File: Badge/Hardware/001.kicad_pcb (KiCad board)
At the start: 2 copper layers, 92.2 x 84.3 mm, 3 parts

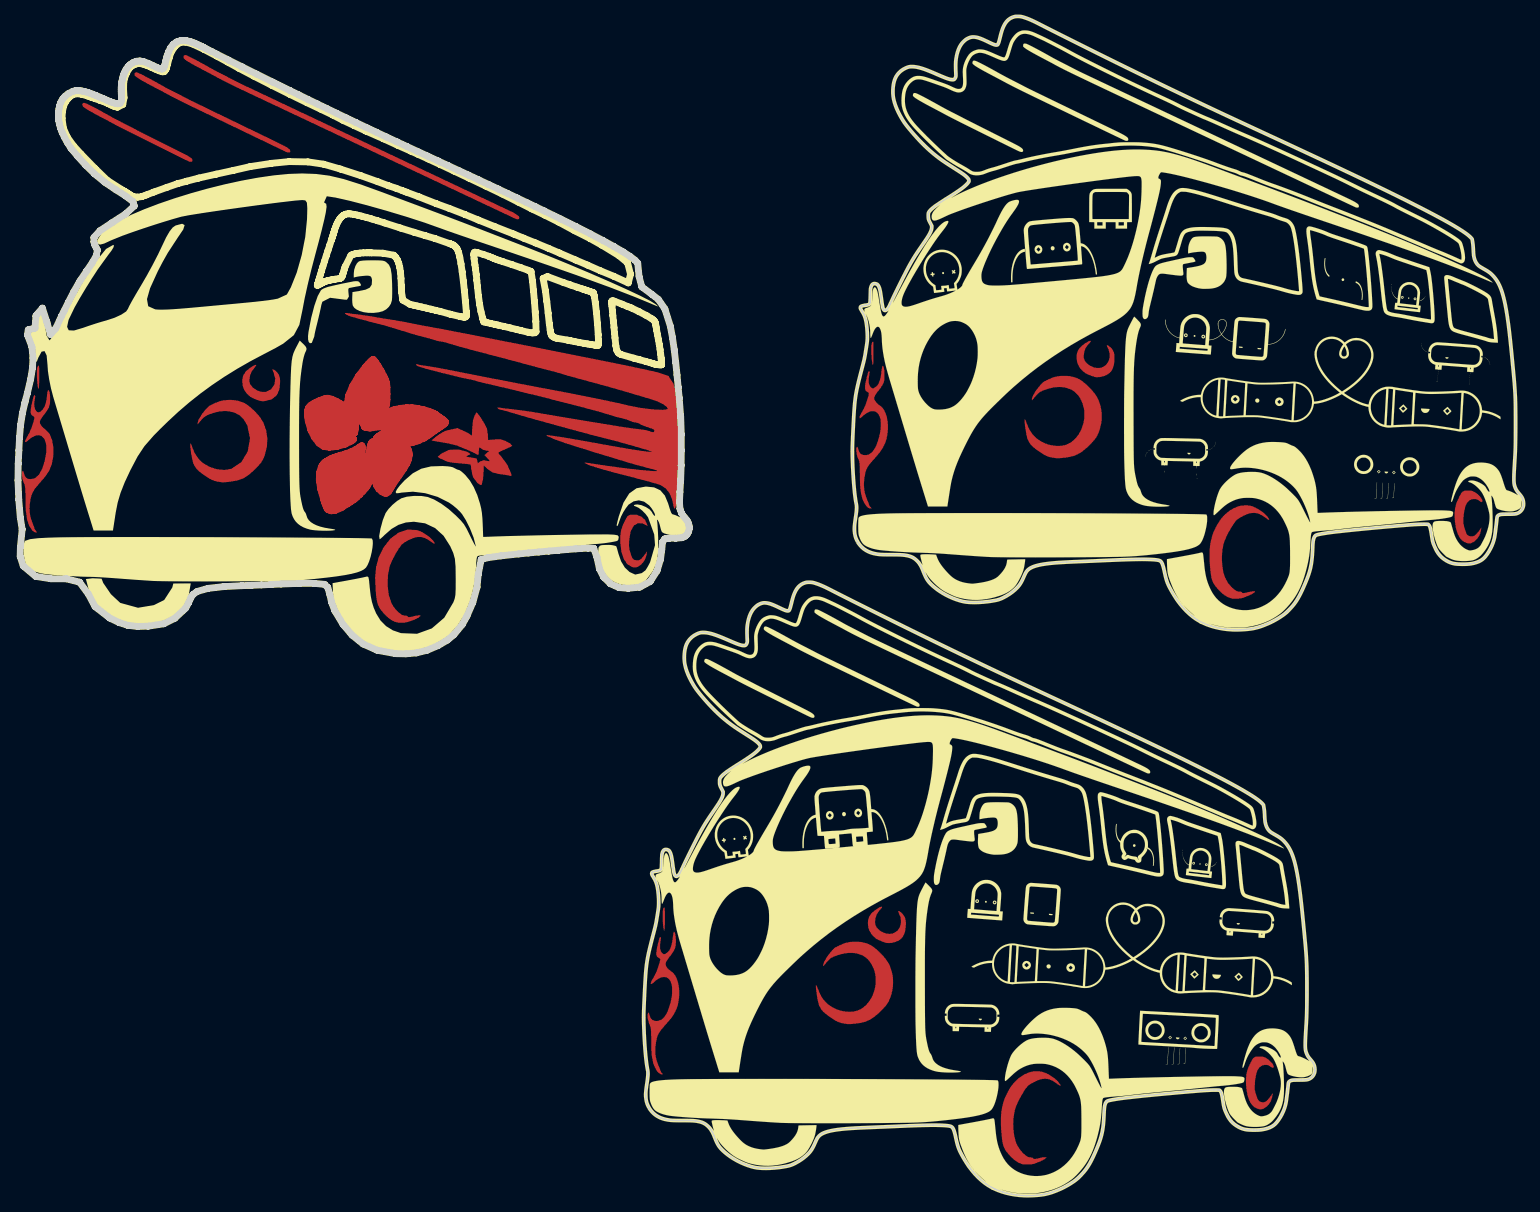
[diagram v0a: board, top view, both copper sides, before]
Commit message: Updates
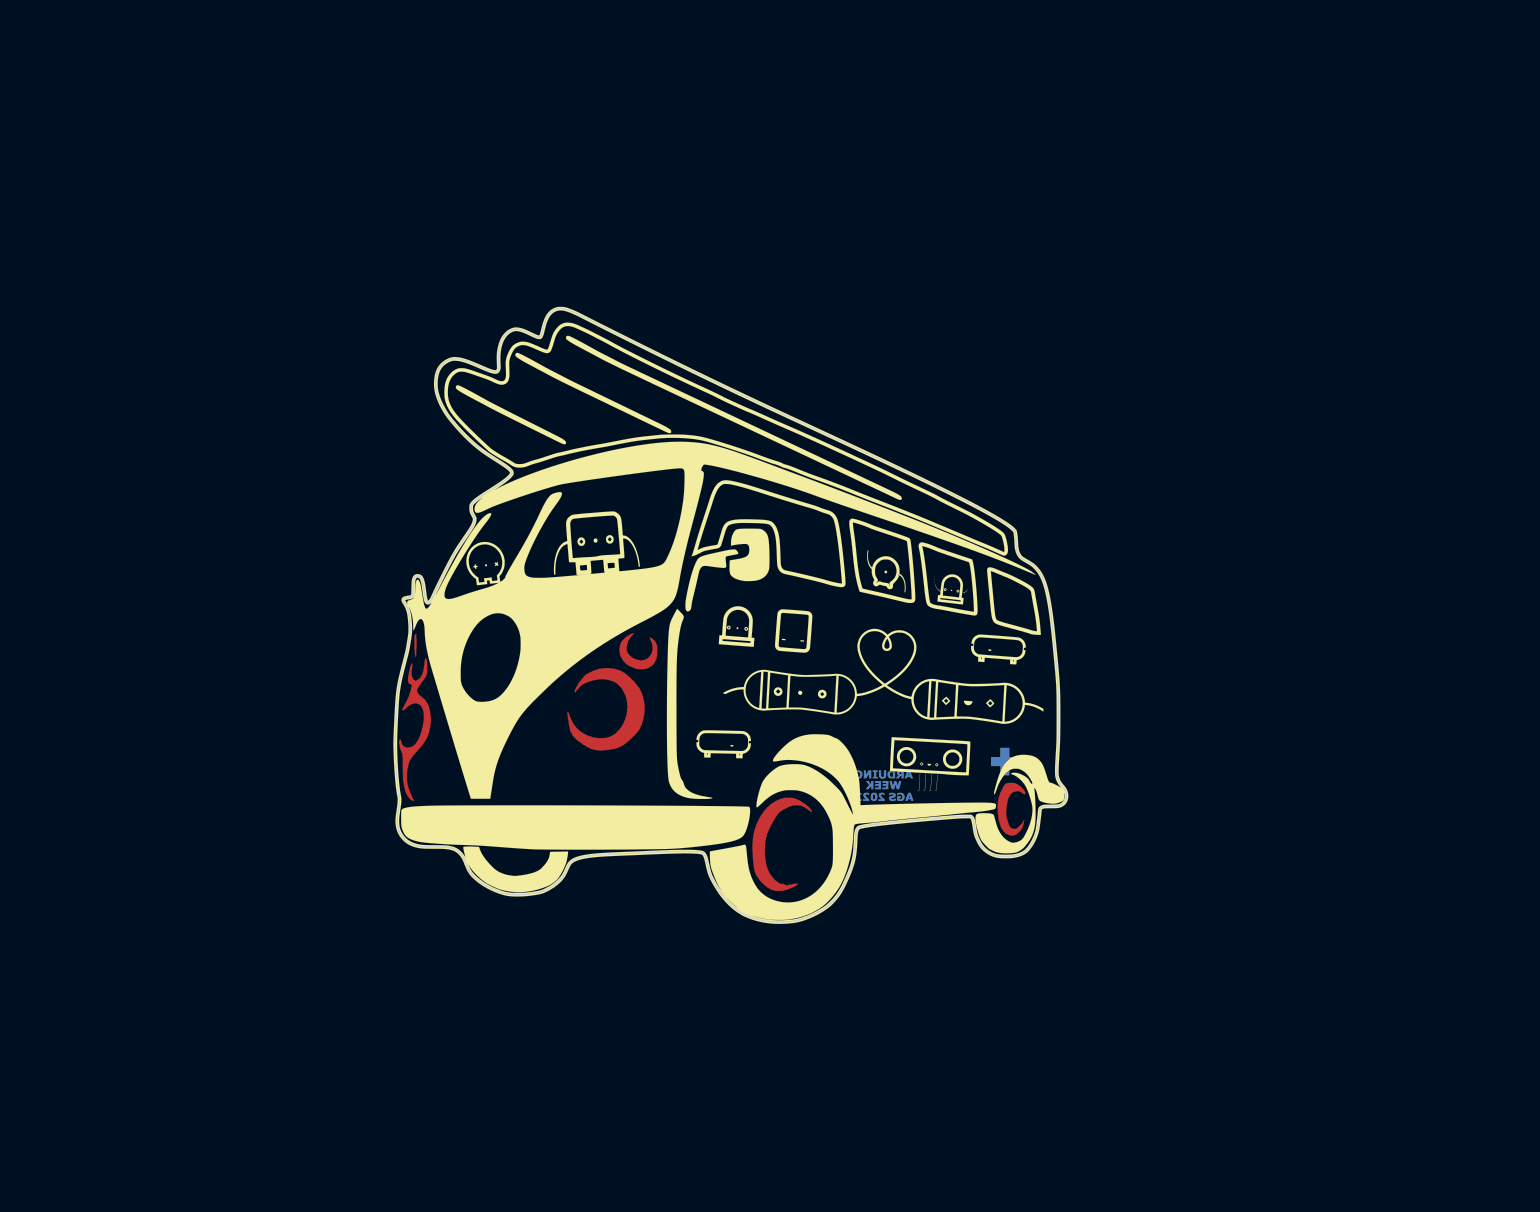
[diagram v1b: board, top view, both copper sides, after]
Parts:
- removed the Ref** at (203.7, 55.1)
- removed svg2mod: G***, combi:Combi.All.03
- added Ref**: Val**, combi:logo_AGS_2022, F.Cu at (172.7, 118.1)
- moved Ref** 50.7 mm to (141.0, 95.2)

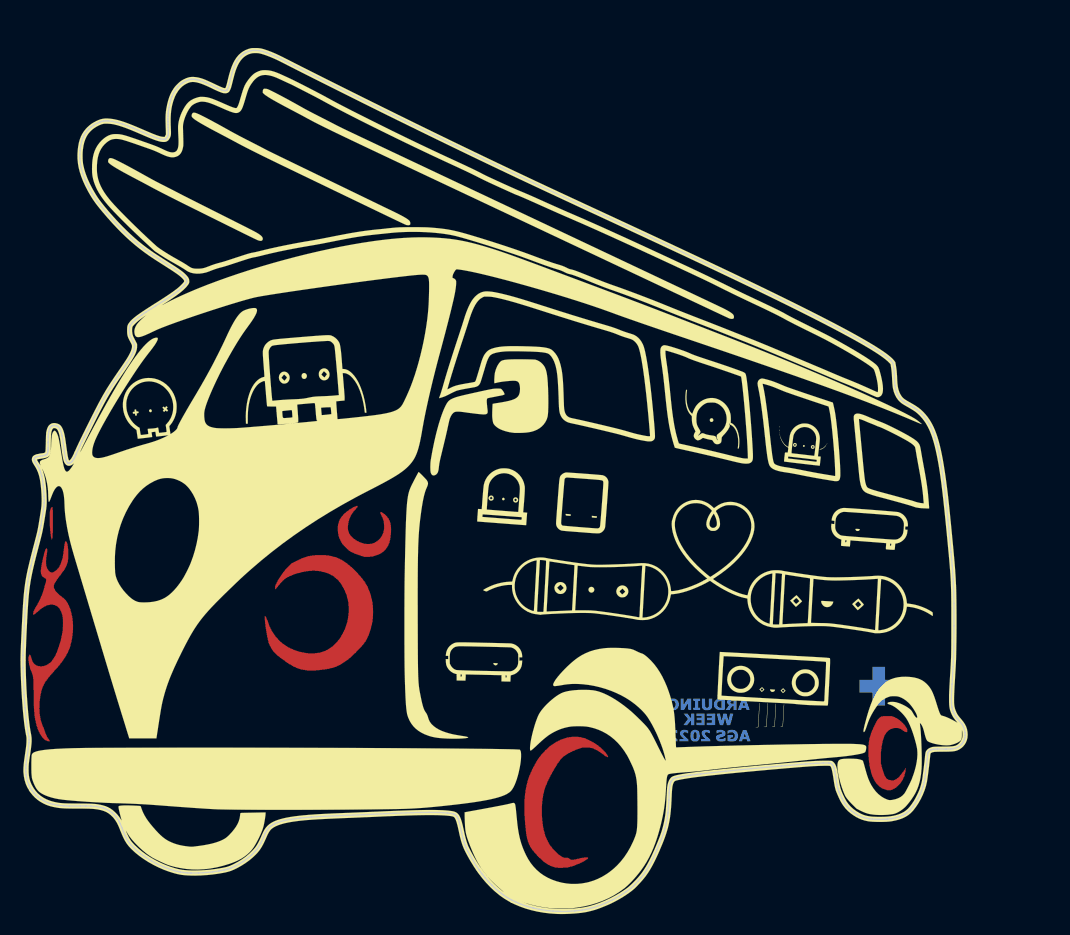
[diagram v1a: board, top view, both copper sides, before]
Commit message: Update Combi 4
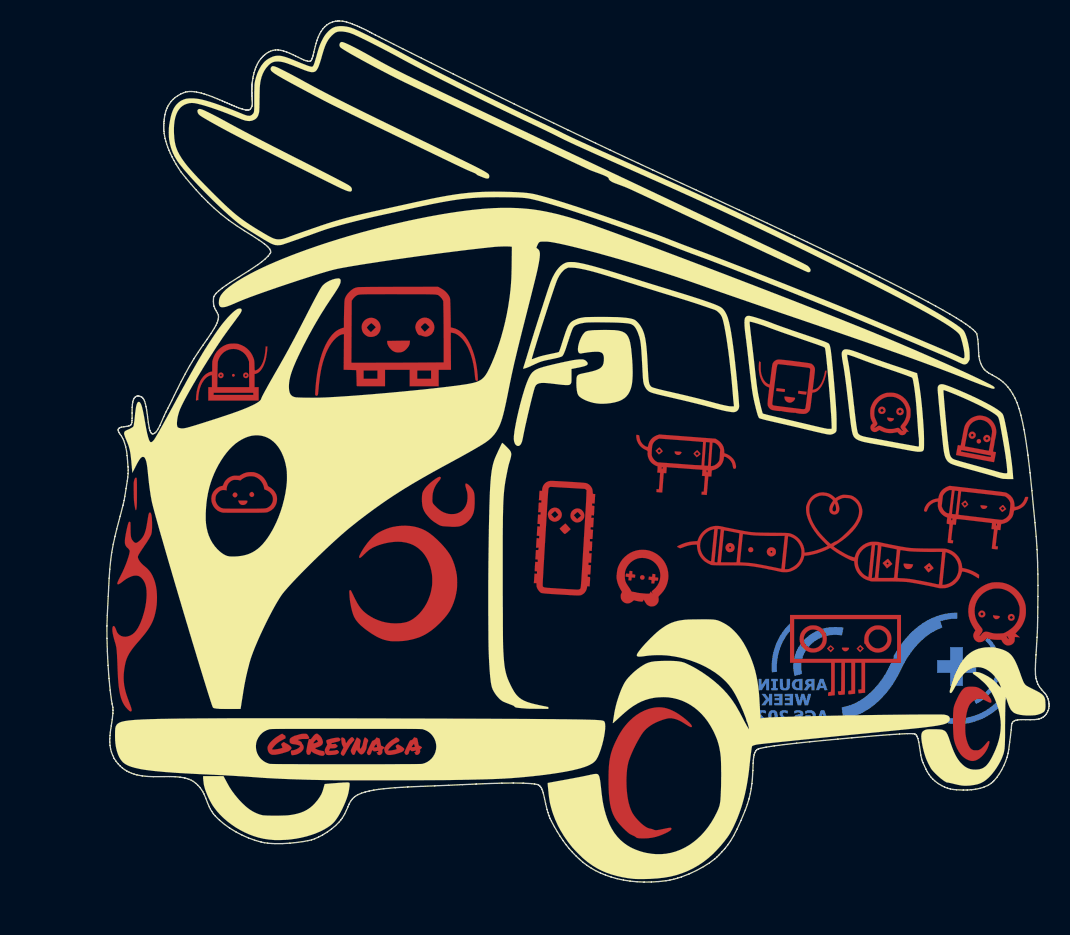
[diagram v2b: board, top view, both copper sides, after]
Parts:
- removed the Ref** at (141.0, 95.2)
- added Ref**: Val**, combi:Combi_4, F.Cu at (147.3, 94.0)
- moved Ref** 7.86 mm to (180.3, 116.2)
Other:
- outline, holes or cut-outs redrawn
